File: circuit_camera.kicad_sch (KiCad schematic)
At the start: 22 parts, among them U11 LM2576HVS-5, U12 LDO 5-3.3V-(MIC5504-3.3YM5-TR)

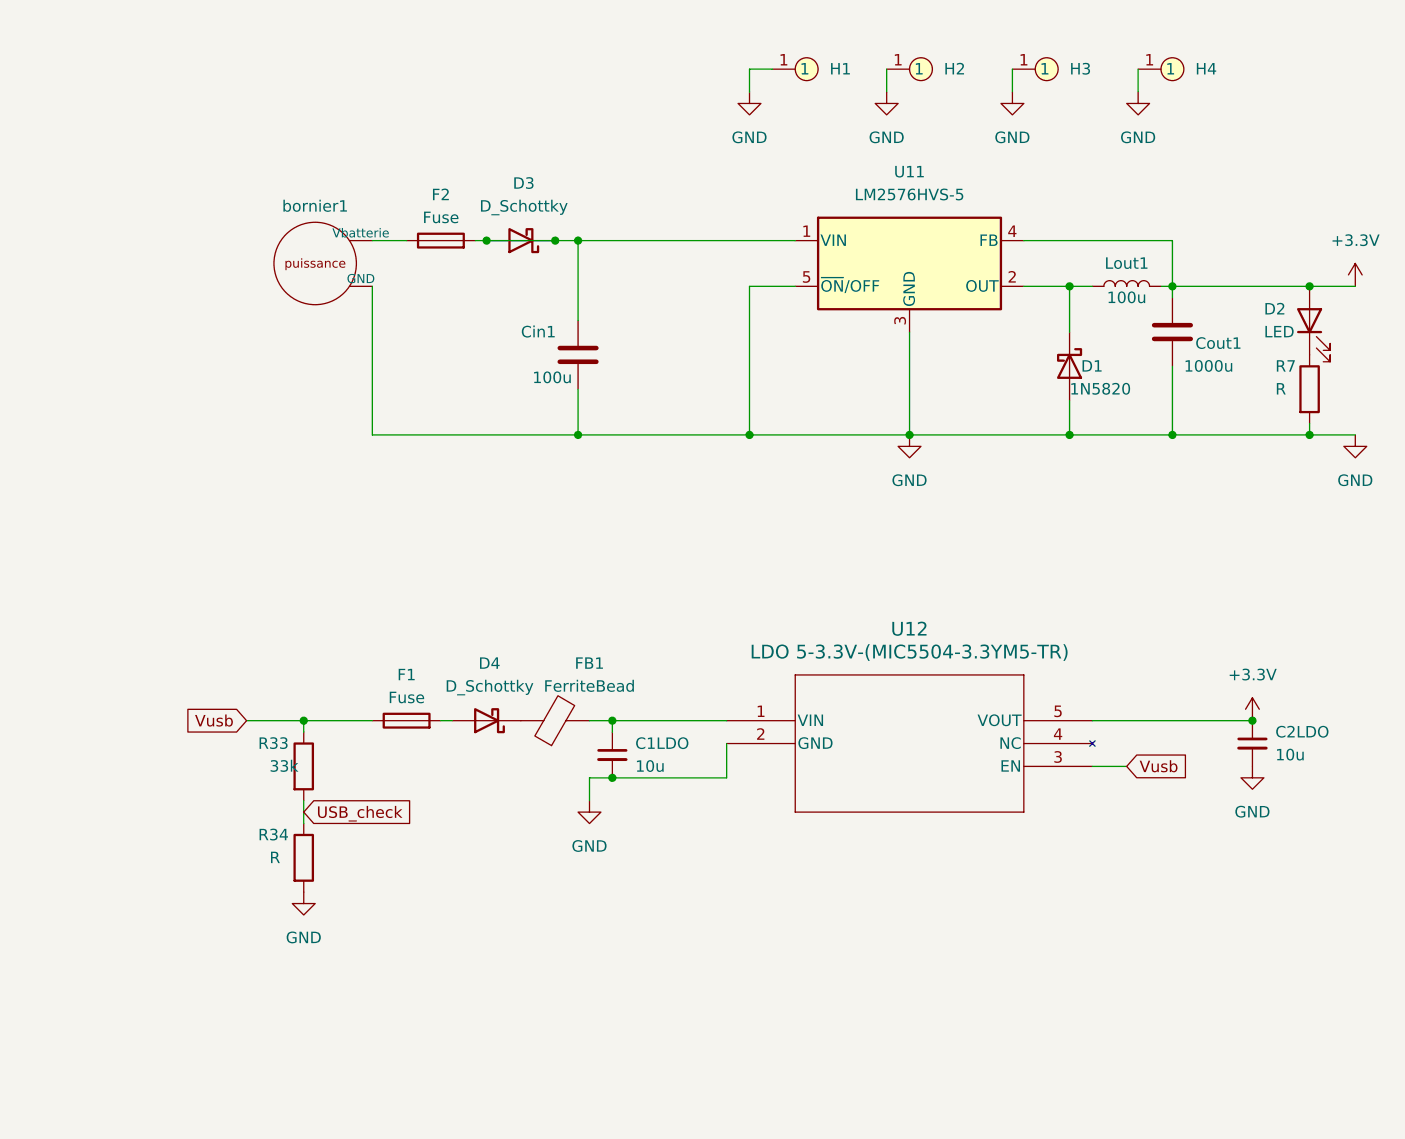
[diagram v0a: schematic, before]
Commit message: Schematic fini, en théorie
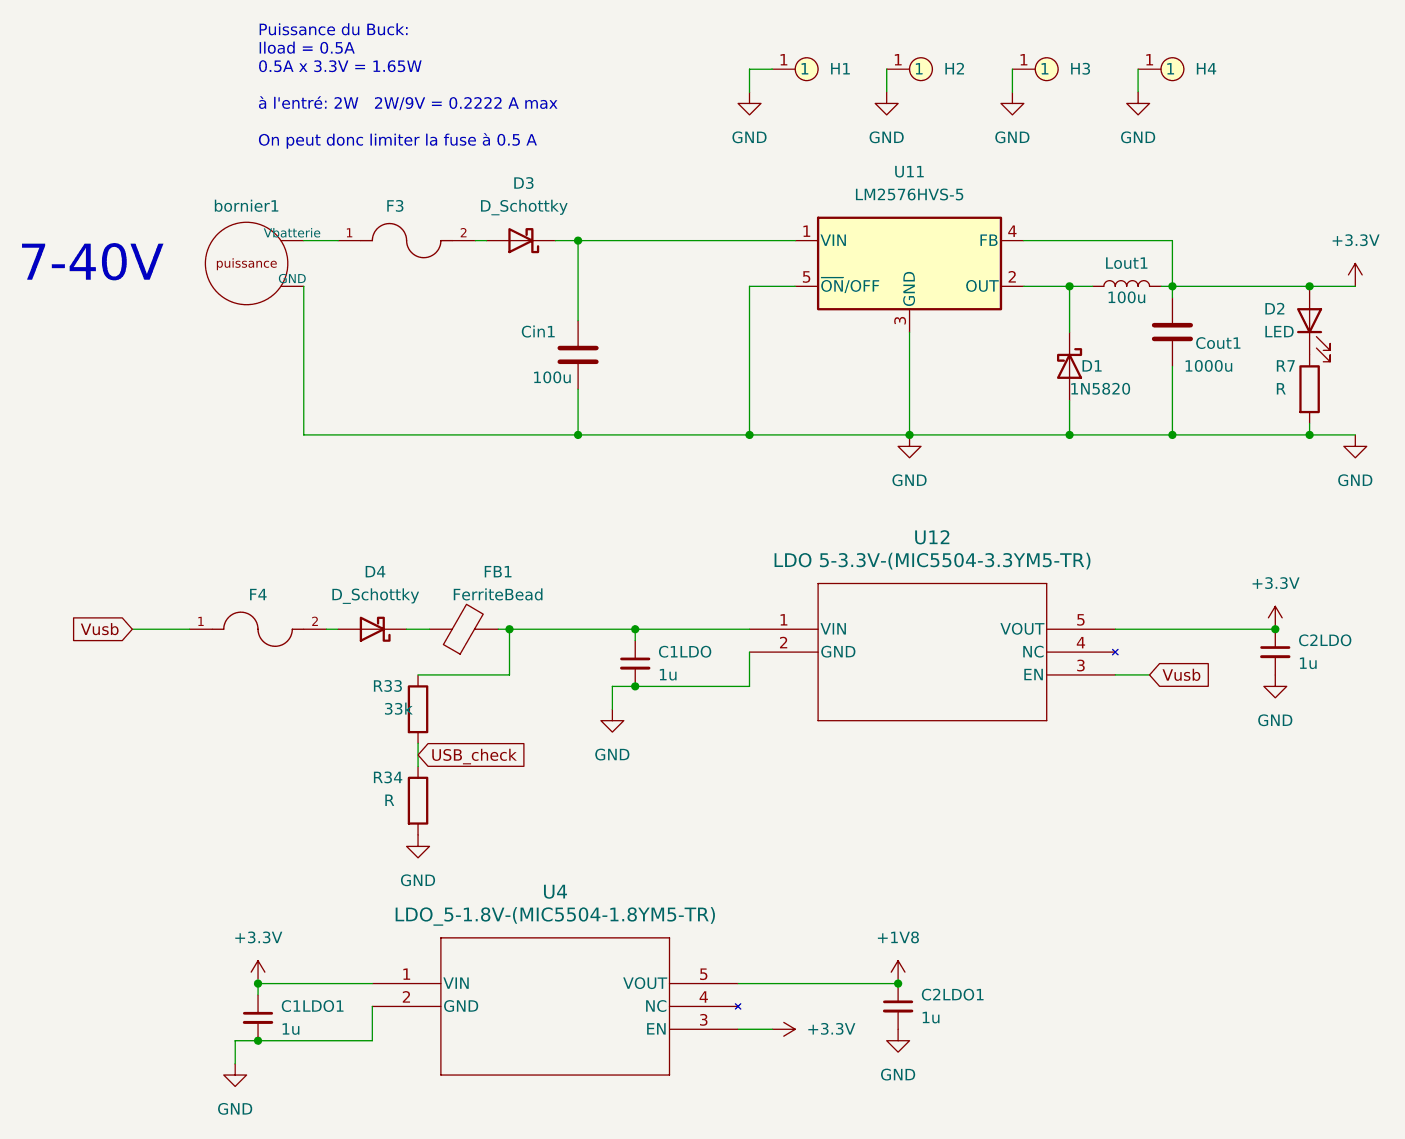
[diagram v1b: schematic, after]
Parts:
- removed F1, F2: Fuse, symbol Device:Fuse
- added C1LDO1, C2LDO1: 1u, symbol Device:C_Small
- added F3, F4: PTC_resettable_fuse_(MF-MSMF030-2), MF-MSMF030-2:FUSER_MF-MSMF030-2, symbol GAUL-Symboles:PTC_resettable_fuse_(MF-MSMF030-2)
- added U4: LDO_5-1.8V-(MIC5504-1.8YM5-TR), SOT-23-5_MC_MCH, symbol GAUL-Symboles:LDO_5-1.8V-(MIC5504-1.8YM5-TR)
- C1LDO, C2LDO: value 10u -> 1u
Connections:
- net +3.3V: now also C1LDO1.1, U4.1 (VIN), U4.3 (EN)
- net GND: now also C1LDO1.2, C2LDO1.2, U4.2 (GND)
- net Vusb: now also F4.1; no longer R33.1
- net at bornier1.1 (Vbatterie): now also F3.1
- net at C1LDO.1, FB1.2, U12.1 (VIN): now also R33.1
- net at Cin1.1, D3.1 (K), U11.1 (VIN): no longer D3.2 (A)
- net at D4.2 (A): now also F4.2
- new net: D3.2 (A), F3.2
- new net +1V8: C2LDO1.1, U4.5 (VOUT)
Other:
- note added: "7-40V"
- note added: "Puissance du Buck: Iload = 0.5A 0.5A x 3.3V = 1.65W à l'entré: 2W 2W/9V = 0.2222 A max On peut donc limiter la fuse à 0.5 A"
- moved on the sheet: C1LDO, C2LDO, D4, FB1, R33, R34, U12, bornier1
